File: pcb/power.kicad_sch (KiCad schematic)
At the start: 12 parts, among them J2 USB_C_Receptacle_USB2.0_14P, J3 Conn_01x02, J6 Conn_01x02, U2 nPM1300-QEXX

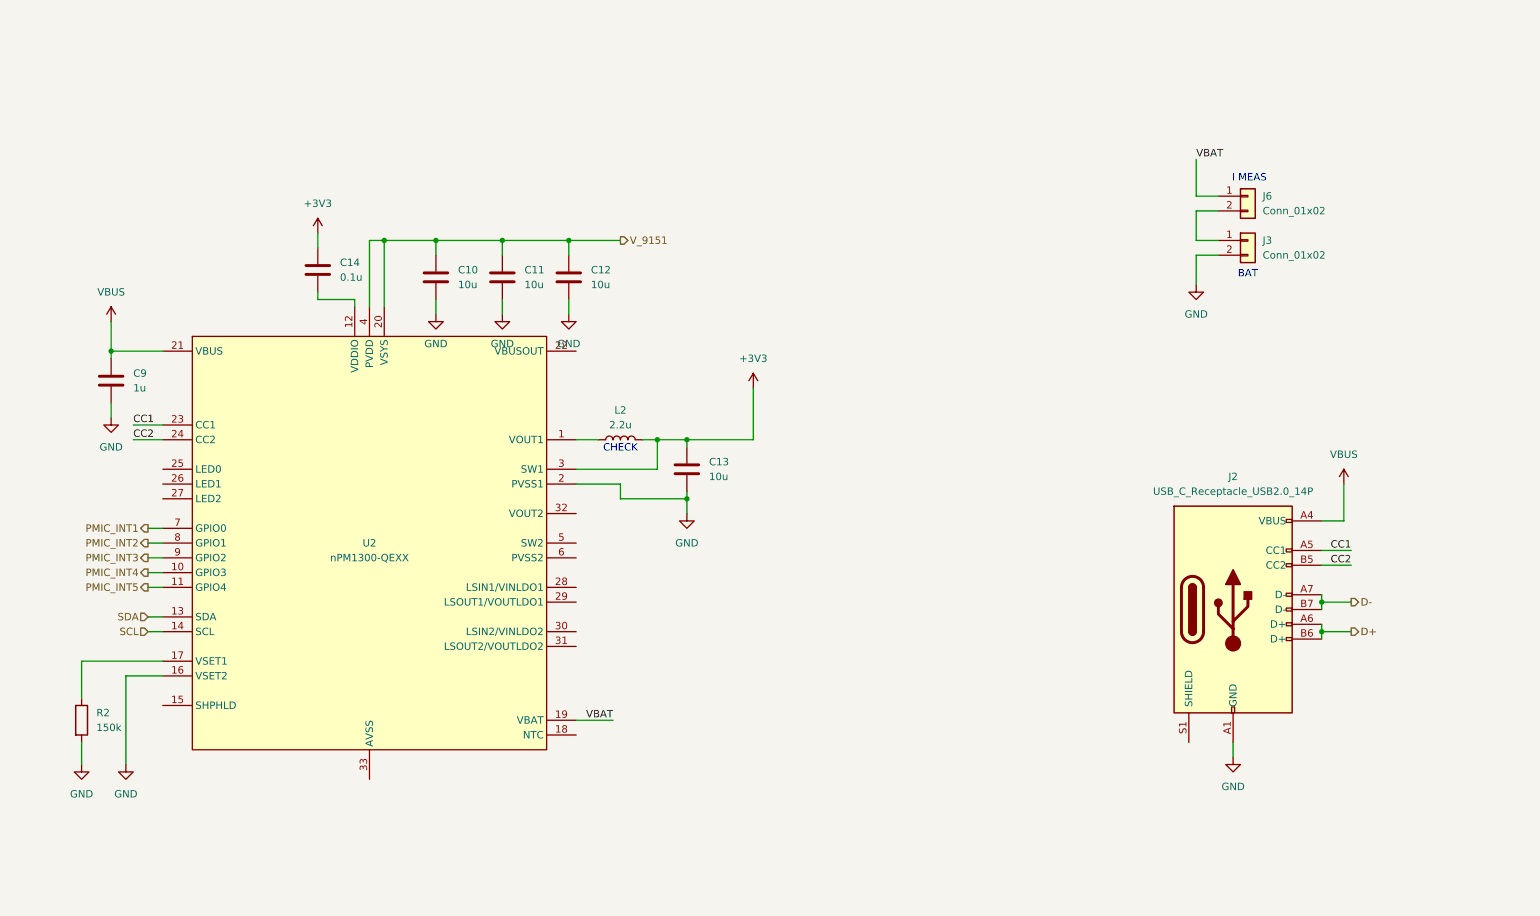
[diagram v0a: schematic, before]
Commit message: Clean up sch
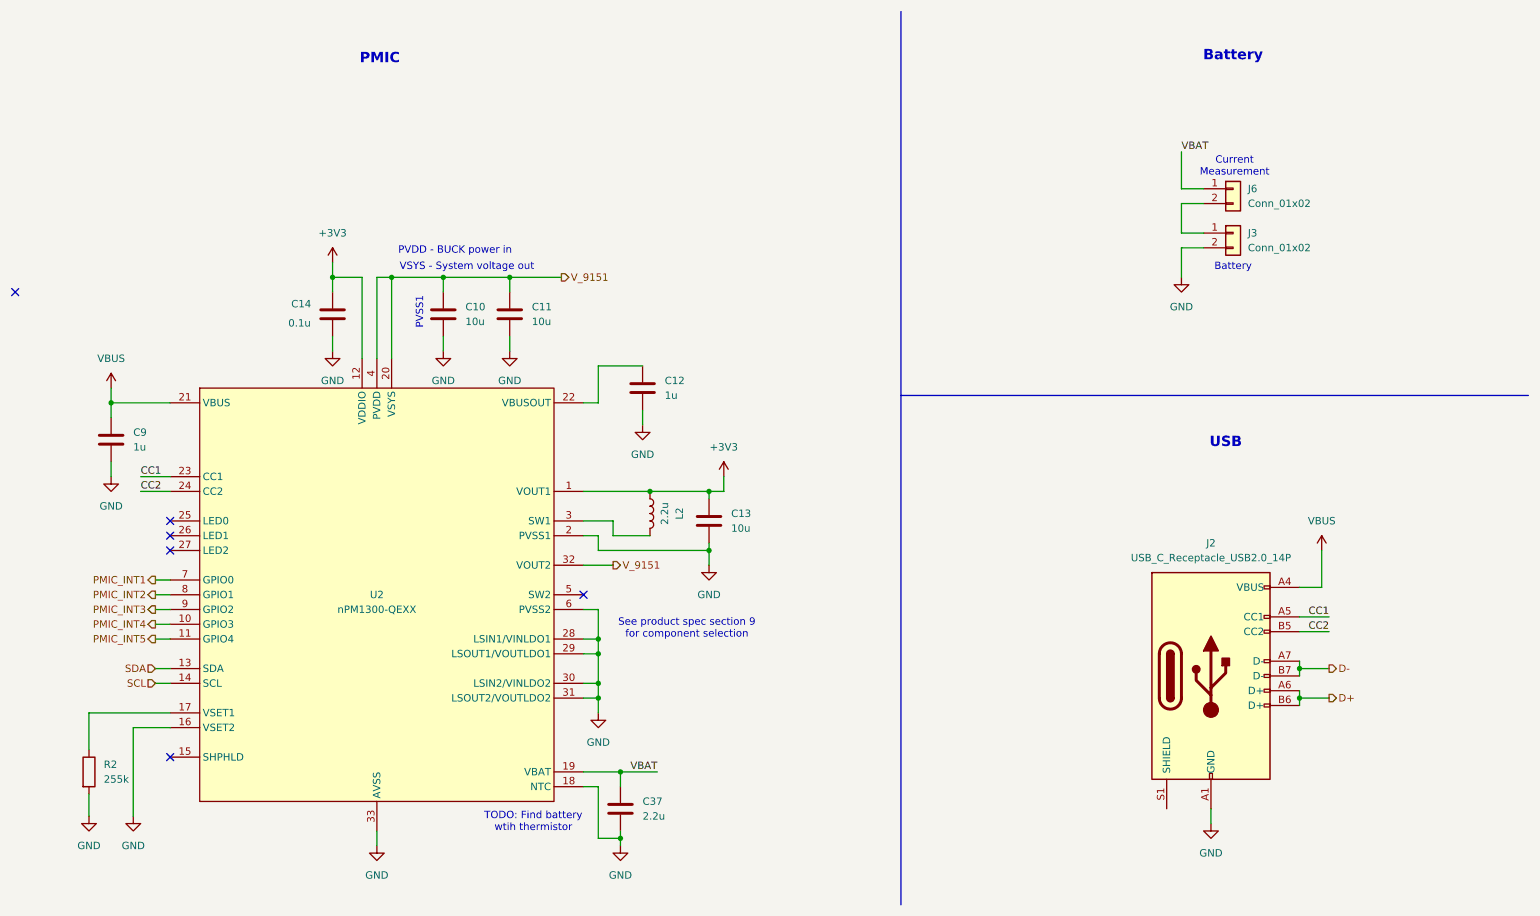
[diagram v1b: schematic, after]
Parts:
- added C37: 2.2u, symbol Device:C
- C12: value 10u -> 1u
- R2: value 150k -> 255k
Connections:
- net +3V3: now also L2.1, U2.1 (VOUT1), U2.12 (VDDIO); no longer L2.2, U2.3 (SW1)
- net GND: now also C14.2, U2.18 (NTC), U2.28 (LSIN1/VINLDO1), U2.29 (LSOUT1/VOUTLDO1), U2.30 (LSIN2/VINLDO2), U2.31 (LSOUT2/VOUTLDO2), U2.33 (AVSS), U2.6 (PVSS2), C37.2
- net VBAT: now also C37.1
- net V_9151: now also U2.32 (VOUT2); no longer C12.1
- net at U2.22 (VBUSOUT): now also C12.1
- new net: L2.2, U2.3 (SW1)
- no-connect marks 0 -> 6
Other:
- note added: "Battery"
- note added: "Current Measurement"
- note added: "PMIC"
- note added: "PVDD - BUCK power in"
- note added: "PVSS1"
- note added: "See product spec section 9 for component selection"
- note added: "TODO: Find battery wtih thermistor"
- note added: "USB"
- note added: "VSYS - System voltage out"
- note removed: "BAT"
- note removed: "CHECK"
- note removed: "I MEAS"
- moved on the sheet: C10, C11, C13, C14, C9, J2, J3, J6, L2, R2, U2

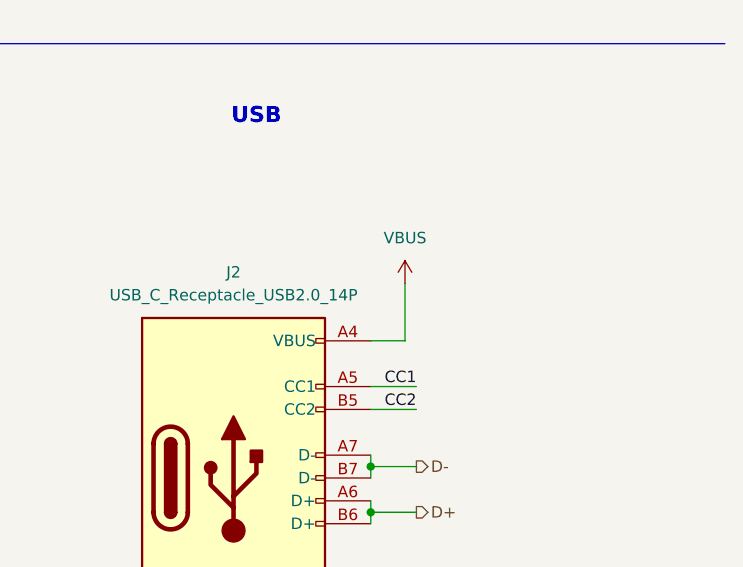
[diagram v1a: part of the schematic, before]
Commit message: Footprints
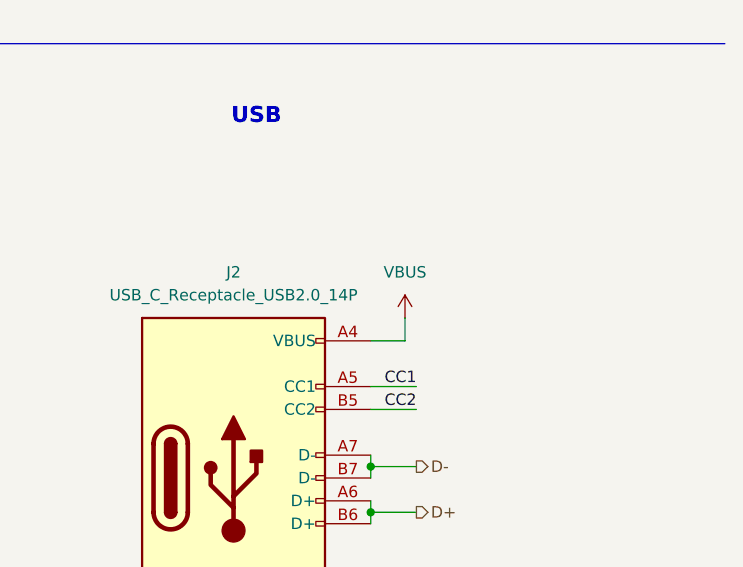
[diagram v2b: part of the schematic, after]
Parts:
- C10, C11, C13: footprint (none) -> Capacitor_SMD:C_0805_2012Metric
- C12, C14, C37, C9, L2: footprint (none) -> Capacitor_SMD:C_0603_1608Metric
- J2: footprint (none) -> Connector_USB:USB_C_Receptacle_GCT_USB4105-xx-A_16P_TopMnt_Horizontal
- J3: footprint (none) -> Connector_JST:JST_SHL_SM02B-SHLS-TF_1x02-1MP_P1.00mm_Horizontal
- J6: footprint (none) -> Connector_PinHeader_2.54mm:PinHeader_1x02_P2.54mm_Vertical
- R2: footprint (none) -> Resistor_SMD:R_0603_1608Metric
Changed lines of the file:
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@@
-	(wire
-		(pts
-			(xy 248.92 105.41) (xy 248.92 111.76)
-		)
-		(stroke
-			(width 0)
-			(type default)
-		)
-	)
 	(wire
 		(pts
@@
 		(pts
 			(xy 121.92 123.19) (xy 124.46 123.19)
+		)
+		(stroke
+			(width 0)
+			(type default)
+		)
+	)
+	(wire
+		(pts
+			(xy 248.92 109.22) (xy 248.92 111.76)
 		)
 		(stroke
@@
 			)
 		)
-		(property "Footprint" ""
+		(property "Footprint" "Connector_PinHeader_2.54mm:PinHeader_1x02_P2.54mm_Vertical"
 			(at 233.68 43.18 0)
 			(effects
@@
 			)
 		)
-		(property "Footprint" ""
+		(property "Footprint" "Connector_JST:JST_SHL_SM02B-SHLS-TF_1x02-1MP_P1.00mm_Horizontal"
 			(at 233.68 50.8 0)
 			(effects
@@
 			)
 		)
-		(property "Footprint" ""
+		(property "Footprint" "Capacitor_SMD:C_0603_1608Metric"
 			(at 129.2352 153.67 0)
 			(effects
@@
 			)
 		)
-		(property "Footprint" ""
+		(property "Footprint" "Connector_USB:USB_C_Receptacle_GCT_USB4105-xx-A_16P_TopMnt_Horizontal"
 			(at 233.68 127 0)
 			(effects
@@
 			)
 		)
-		(property "Footprint" ""
+		(property "Footprint" "Capacitor_SMD:C_0603_1608Metric"
 			(at 133.0452 81.28 0)
 			(effects
@@
 			)
 		)
-		(property "Footprint" ""
+		(property "Footprint" "Capacitor_SMD:C_0805_2012Metric"
 			(at 144.4752 104.14 0)
 			(effects
@@
 			)
 		)
-		(property "Footprint" ""
+		(property "Footprint" "Capacitor_SMD:C_0603_1608Metric"
 			(at 133.35 99.06 0)
 			(effects
@@
 			)
 		)
-		(property "Footprint" ""
+		(property "Footprint" "Capacitor_SMD:C_0805_2012Metric"
 			(at 110.1852 68.58 0)
 			(effects
@@
 	(symbol
 		(lib_id "power:VBUS")
-		(at 248.92 105.41 0)
+		(at 248.92 109.22 0)
 		(unit 1)
 		(exclude_from_sim no)
@@
 		(fields_autoplaced yes)
 		(property "Reference" "#PWR014"
+			(at 248.92 113.03 0)
+			(effects
+				(font
+					(size 1.27 1.27)
+				)
+				(hide yes)
+			)
+		)
+		(property "Value" "VBUS"
+			(at 248.92 104.14 0)
+			(effects
+				(font
+					(size 1.27 1.27)
+				)
+			)
+		)
+		(property "Footprint" ""
 			(at 248.92 109.22 0)
 			(effects
@@
 			)
 		)
-		(property "Value" "VBUS"
-			(at 248.92 100.33 0)
-			(effects
-				(font
-					(size 1.27 1.27)
-				)
-			)
-		)
-		(property "Footprint" ""
-			(at 248.92 105.41 0)
-			(effects
-				(font
-					(size 1.27 1.27)
-				)
-				(hide yes)
-			)
-		)
 		(property "Datasheet" ""
-			(at 248.92 105.41 0)
+			(at 248.92 109.22 0)
 			(effects
 				(font
@@
 		)
 		(property "Description" "Power symbol creates a global label with name \"VBUS\""
-			(at 248.92 105.41 0)
+			(at 248.92 109.22 0)
 			(effects
 				(font
@@
 			)
 		)
-		(property "Footprint" ""
+		(property "Footprint" "Resistor_SMD:R_0603_1608Metric"
 			(at 35.052 143.51 90)
 			(effects
@@
 			)
 		)
-		(property "Footprint" ""
+		(property "Footprint" "Capacitor_SMD:C_0603_1608Metric"
 			(at 79.7052 68.58 0)
 			(effects
@@
 			)
 		)
-		(property "Footprint" ""
+		(property "Footprint" "Capacitor_SMD:C_0805_2012Metric"
 			(at 98.7552 68.58 0)
 			(effects
@@
 			)
 		)
-		(property "Footprint" ""
+		(property "Footprint" "Capacitor_SMD:C_0603_1608Metric"
 			(at 41.6052 90.17 0)
 			(effects
